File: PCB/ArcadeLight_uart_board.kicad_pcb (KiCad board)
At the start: 2 copper layers, 52.4 x 77.1 mm, 20 parts, among them J1 Partition_Lights_L, J10 Circle_LED, J11 Cross_LED, J12 Square_LED, J13 Triangle_LED, J3 12V_In, J9 Partition_Lights_R, P7 CONN_01X01, P9 CONN_01X01, Q1 AO3404A, Q2 IRFR9024N, U1 Arduino_Nano_v3.x, U2 ULN2003, U3 ULN2003

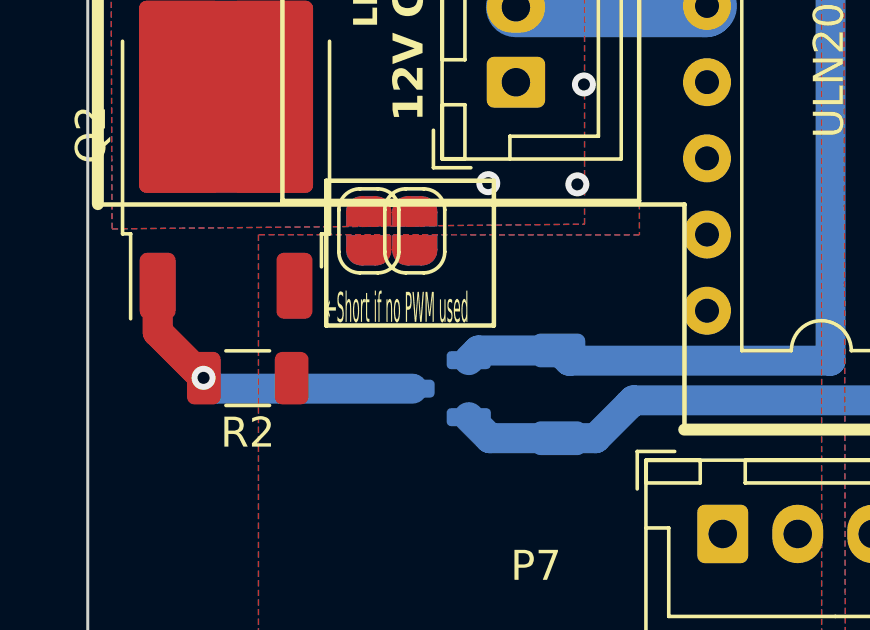
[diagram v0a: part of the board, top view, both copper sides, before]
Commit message: Readme update
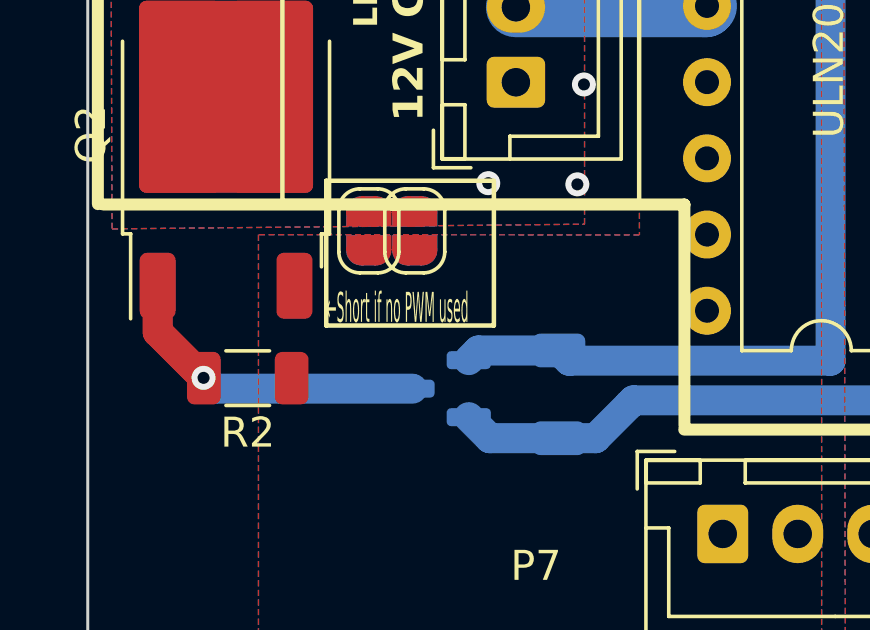
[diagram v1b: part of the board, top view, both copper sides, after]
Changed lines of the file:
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@@
     (stroke (width 0.15) (type default)) (fill none) (layer "F.SilkS"))
   (gr_line (start 192.151 97.282) (end 201.93 97.282)
-    (stroke (width 0.15) (type default)) (layer "F.SilkS"))
+    (stroke (width 0.4) (type default)) (layer "F.SilkS"))
   (gr_rect (start 188.528 69.222) (end 200.42 97.162)
     (stroke (width 0.15) (type default)) (fill none) (layer "F.SilkS"))
@@
     (stroke (width 0.4) (type default)) (layer "F.SilkS"))
   (gr_line (start 201.93 97.282) (end 201.93 104.648)
-    (stroke (width 0.15) (type default)) (layer "F.SilkS"))
+    (stroke (width 0.4) (type default)) (layer "F.SilkS"))
   (gr_line (start 231.648 98.552) (end 231.648 104.76)
     (stroke (width 0.4) (type default)) (layer "F.SilkS"))
@@
     (stroke (width 0.4) (type default)) (layer "F.SilkS"))
   (gr_line (start 182.5625 97.282) (end 192.3415 97.282)
-    (stroke (width 0.15) (type default)) (layer "F.SilkS"))
+    (stroke (width 0.4) (type default)) (layer "F.SilkS"))
   (gr_rect (start 182.04 40.462) (end 234.41 117.545)
     (stroke (width 0.1) (type default)) (fill none) (layer "Edge.Cuts"))
